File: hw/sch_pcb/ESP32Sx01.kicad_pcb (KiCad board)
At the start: 2 copper layers, 60.5 x 50.3 mm, 32 parts, among them J1 HEADER_1x03, J2 USBC_USB4105-GF-A, J3 HEADER_1x12, J4 HEADER_1x12, J5 HEADER_1x12, J6 HEADER_1x03, J8 HEADER_2x05, Q1 BC817-25, SW1 434133025816, U1 NCP1117-3.3, U2 USBLC6-2SC6, U3 ESP32-S3-MINI-1, Y1 Crystal_Small

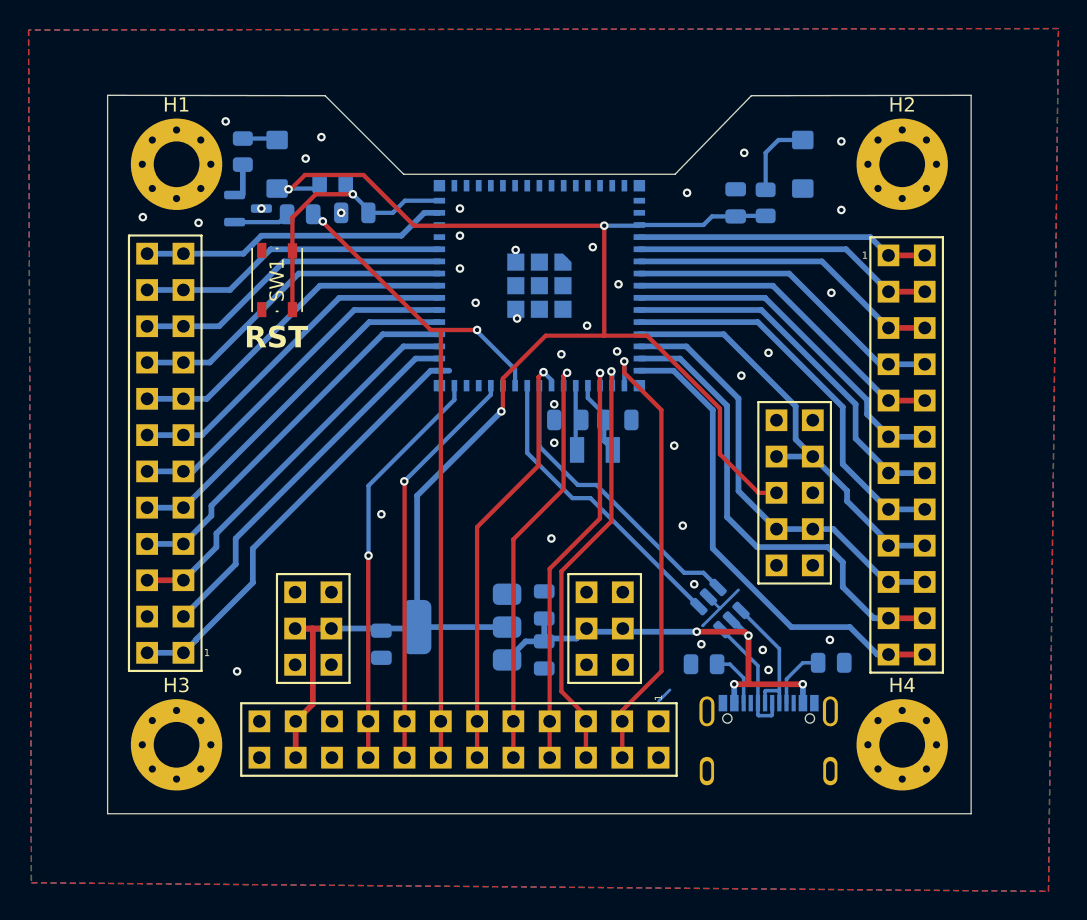
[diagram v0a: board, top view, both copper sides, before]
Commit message: finishing PCB design
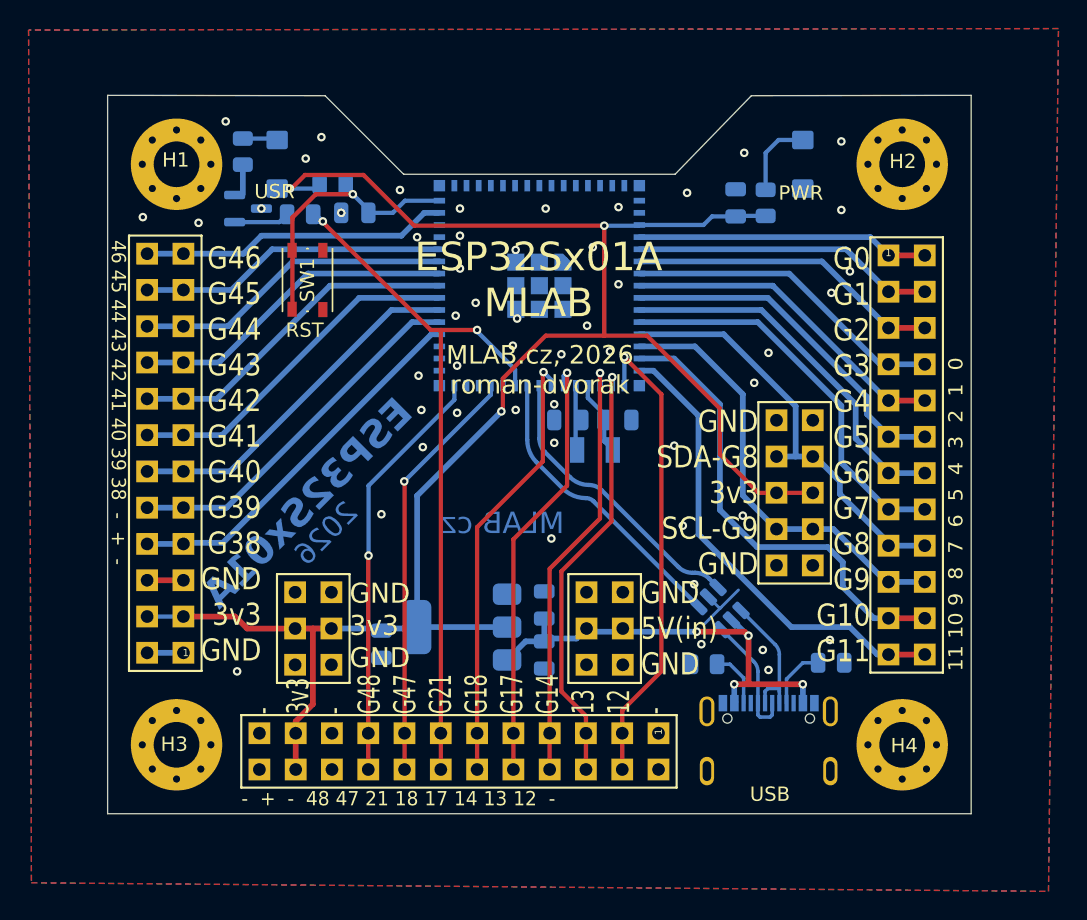
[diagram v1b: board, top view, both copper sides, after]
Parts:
- moved SW1 2.12 mm to (132.3, 92.8), turned to -90 degrees
- moved J4 0.83 mm to (142.9, 125.8)
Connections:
- J5 pad 1: /GPIO35 -> GND
- J5 pad 2: /GPIO35 -> GND
- J5 pad 3: /GPIO36 -> +3V3
- J5 pad 4: /GPIO36 -> +3V3
- J5 pad 5: /GPIO37 -> GND
- J5 pad 6: /GPIO37 -> GND
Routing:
- net /GPIO35: track 30.8 -> 0.00 mm
- net /GPIO37: track 27.8 -> 0.00 mm
- net /GPIO36: track 26.5 -> 0.00 mm
- net +3V3: track 120.2 -> 134.2 mm
- net GND: track 4.74 -> 9.75 mm, vias 37 -> 51
- net /GPIO21: track 49.8 -> 50.6 mm
- net /GPIO17: track 29.5 -> 30.3 mm
- net /GPIO48: track 28.5 -> 29.4 mm
- net /GPIO47: track 28.6 -> 29.4 mm
- net /GPIO18: track 30.1 -> 30.9 mm
- net /GPIO14: track 29.3 -> 30.1 mm
- net /GPIO11: track 33.9 -> 33.1 mm
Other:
- board text added: "- + - 48 47 21 18 17 14 13 12 -"
- board text added: "- 3v3 - G48 G47 G21 G18 G17 G14 13 12 -"
- board text added: "11 10 9 8 7 6 5 4 3 2 1 0"
- board text added: "2026"
- board text added: "46 45 44 43 42 41 40 39 38 - + -"
- board text added: "ESP32Sx01A"
- board text added: "ESP32Sx01A MLAB"
- board text added: "G0 G1 G2 G3 G4 G5 G6 G7 G8 G9 G10 G11"
- board text added: "G46 G45 G44 G43 G42 G41 G40 G39 G38 GND 3v3 GND"
- board text added: "GND 3v3 GND"
- board text added: "GND 5V(in) GND"
- board text added: "GND SDA-G8 3v3 SCL-G9 GND"
- board text added: "MLAB.cz"
- board text added: "MLAB.cz, 2026 roman-dvorak"
- board text added: "PWR"
- board text added: "USB"
- board text added: "USR"
